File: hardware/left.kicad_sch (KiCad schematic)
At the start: 0 parts

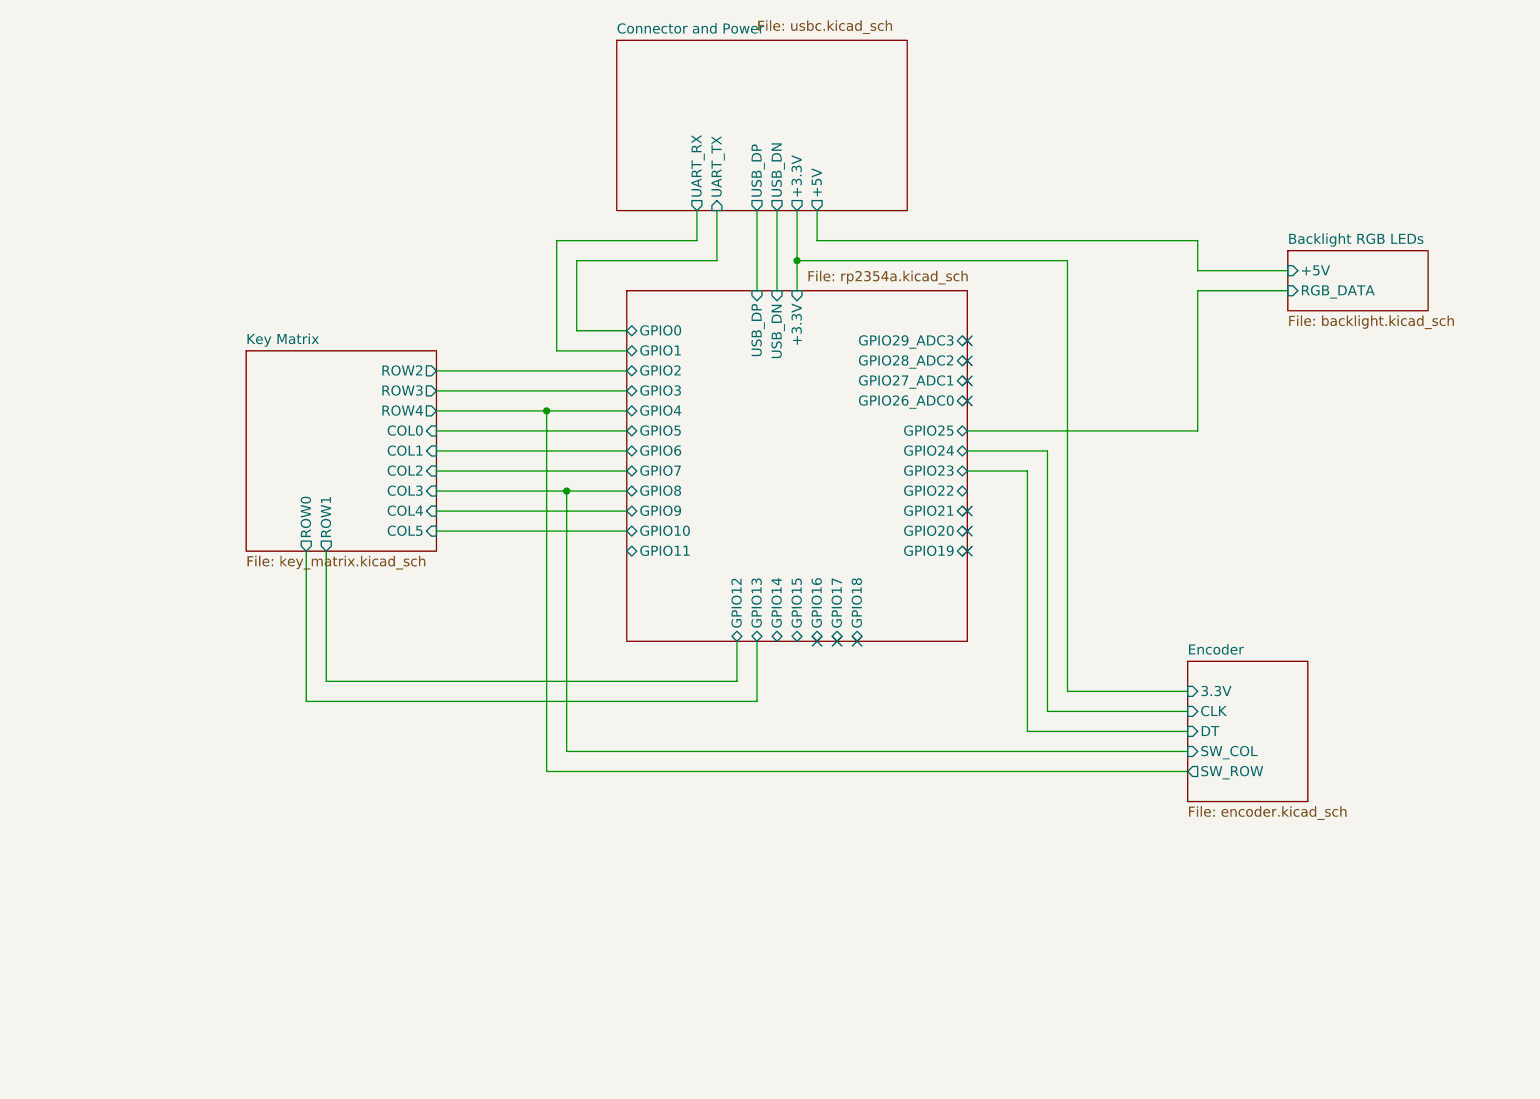
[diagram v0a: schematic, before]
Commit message: electronics
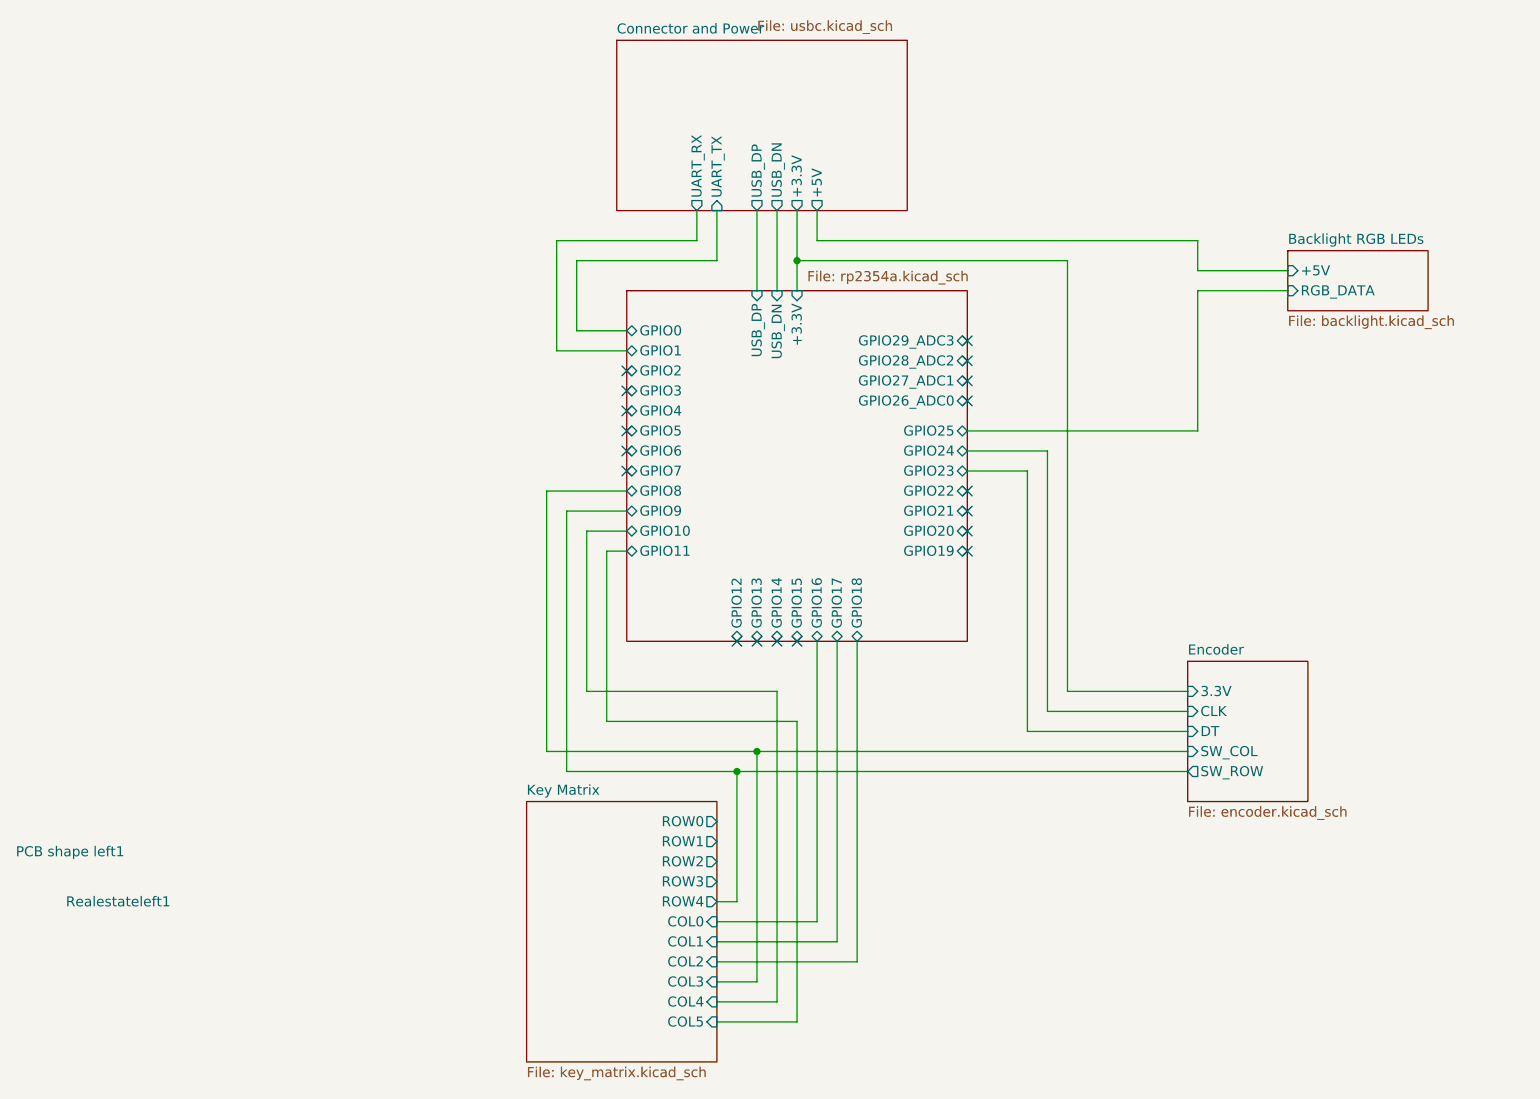
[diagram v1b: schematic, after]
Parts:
- added PCB shape left1: (no value), rp_voyager:PCB left, symbol rp_voyager:PCB_left
- added Realestateleft1: (no value), rp_voyager:Realestate left, symbol rp_voyager:realestate_left
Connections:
- no-connect marks 10 -> 18
